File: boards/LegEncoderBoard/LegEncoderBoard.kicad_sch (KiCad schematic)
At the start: 9 parts, among them J1 Conn_01x05, J2 Conn_01x05, U1 AS5047P-ATST

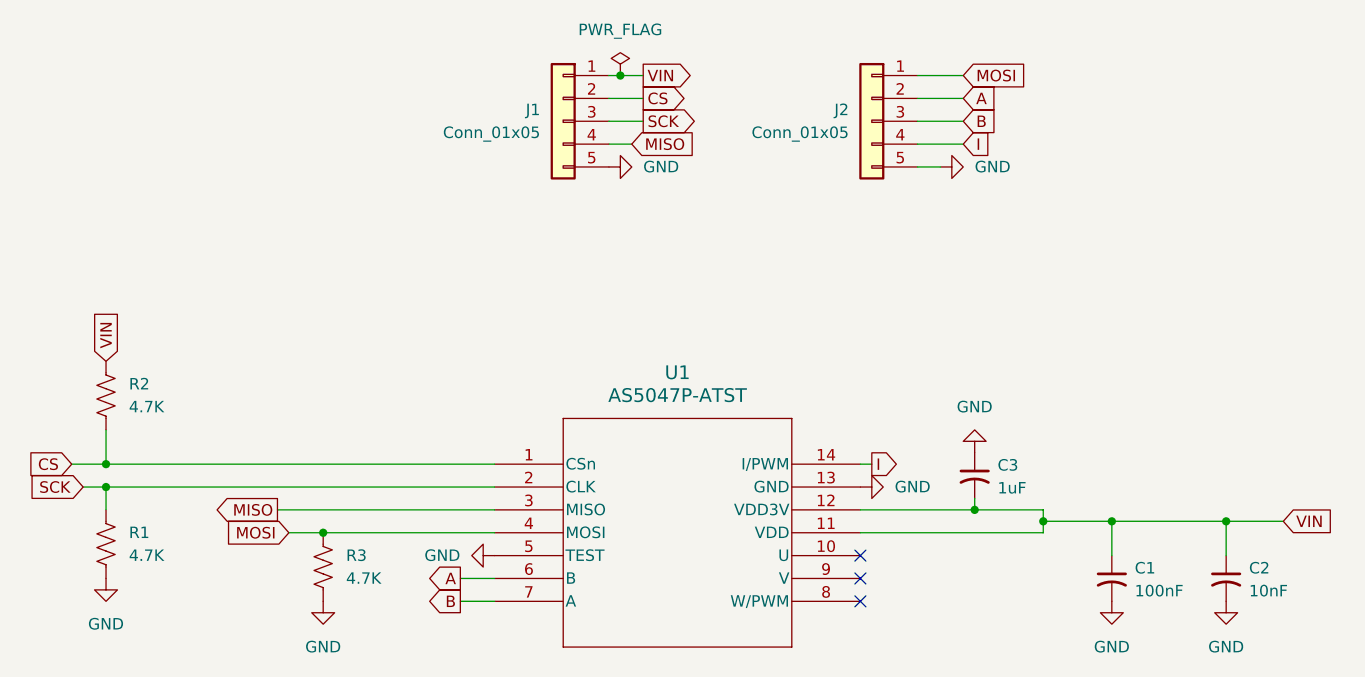
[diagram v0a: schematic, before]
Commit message: Final normalize readme
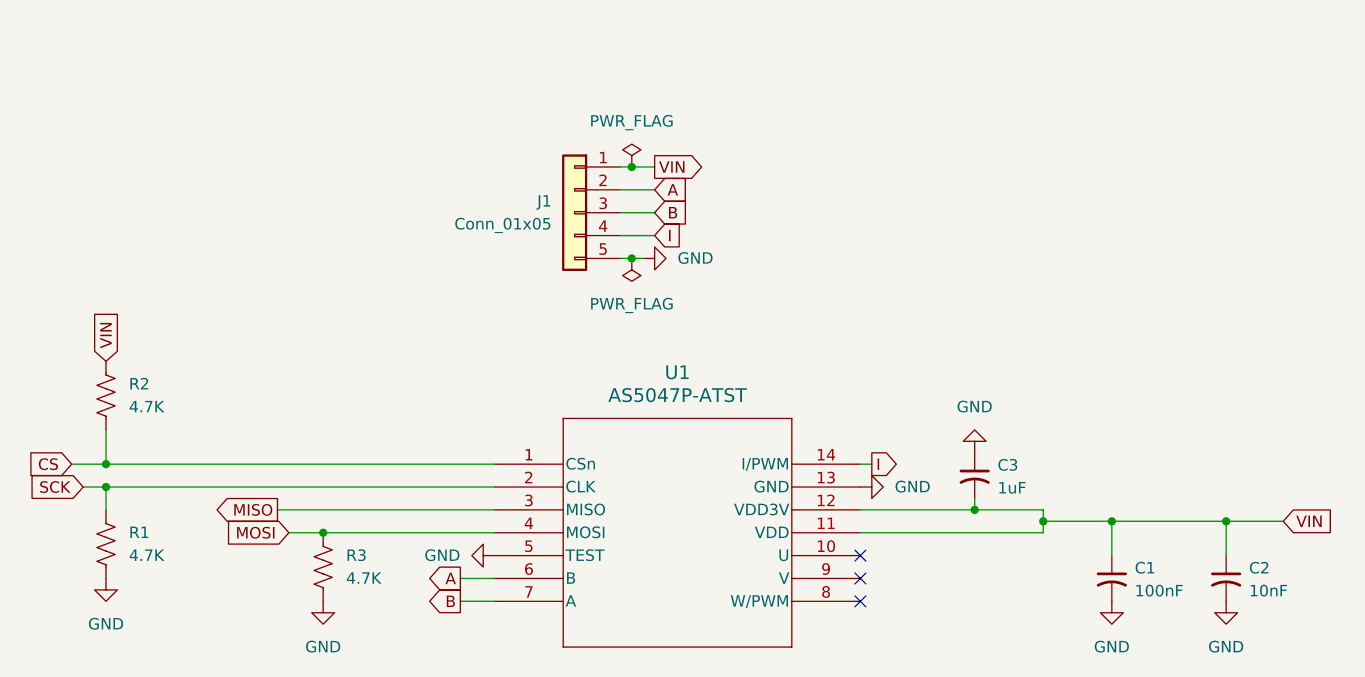
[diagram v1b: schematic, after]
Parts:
- removed J2: Conn_01x05, symbol Connector_Generic:Conn_01x05
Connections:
- net A: now also J1.2 (Pin_2)
- net B: now also J1.3 (Pin_3)
- net CS: no longer J1.2 (Pin_2)
- net I: now also J1.4 (Pin_4)
- net MISO: no longer J1.4 (Pin_4)
- net SCK: no longer J1.3 (Pin_3)
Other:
- moved on the sheet: J1

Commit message: Pre-final leg encoder board
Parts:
- C1: footprint (none) -> Capacitor100nF:885342208002
- C2: footprint (none) -> Capacitor10nF:885012206089
- C3: footprint (none) -> Capacitor1uF:CC0603JRX7R7BB105
- J1: footprint (none) -> Connector_JST:JST_XH_B5B-XH-A_1x05_P2.50mm_Vertical
- R1, R2, R3: footprint (none) -> Resistor4.7K:CR0603-FX-4701ELF
- U1: footprint AS5047P:AS5047P-ATST -> AS5047P-ASST:AS5047P-ASST
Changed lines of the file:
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@@
 			)
 		)
-		(property "Footprint" "AS5047P:AS5047P-ATST"
+		(property "Footprint" "AS5047P-ASST:AS5047P-ASST"
 			(at 110.49 90.17 0)
 			(effects
@@
 			)
 		)
-		(property "Datasheet" "AS5047P-ATST"
+		(property "Datasheet" "AS5047P-ATSM"
 			(at 110.49 90.17 0)
 			(effects
@@
 			)
 		)
-		(property "Footprint" ""
+		(property "Footprint" "Resistor4.7K:CR0603-FX-4701ELF"
 			(at 68.326 82.804 90)
 			(effects
@@
 			)
 		)
-		(property "Footprint" ""
+		(property "Footprint" "Resistor4.7K:CR0603-FX-4701ELF"
 			(at 92.456 101.854 90)
 			(effects
@@
 			)
 		)
-		(property "Footprint" ""
+		(property "Footprint" "Capacitor100nF:885342208002"
 			(at 179.07 102.87 0)
 			(effects
@@
 			)
 		)
-		(property "Footprint" ""
+		(property "Footprint" "Connector_JST:JST_XH_B5B-XH-A_1x05_P2.50mm_Vertical"
 			(at 119.38 62.23 0)
 			(effects
@@
 			)
 		)
-		(property "Footprint" ""
+		(property "Footprint" "Resistor4.7K:CR0603-FX-4701ELF"
 			(at 68.326 99.314 90)
 			(effects
@@
 			)
 		)
-		(property "Footprint" ""
+		(property "Footprint" "Capacitor1uF:CC0603JRX7R7BB105"
 			(at 163.83 91.44 0)
 			(effects
@@
 			)
 		)
-		(property "Footprint" ""
+		(property "Footprint" "Capacitor10nF:885012206089"
 			(at 191.77 102.87 0)
 			(effects
